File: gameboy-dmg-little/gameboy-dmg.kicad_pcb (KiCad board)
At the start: 2 copper layers, 82.5 x 87.5 mm, 83 parts, among them J1 Conn_01x02, J3 Conn_01x08, J5 Raspberry_Pi_2_3, J6 Conn_01x09, J7 USB_B_Micro, J8 Conn_01x02, P1 RK10J_POT, SW1 SW_DIP_x01, U1 MCP23017_SO, U2 TP4056, U3 FS312F-G, U4 FS8205, U5 MT3608, U6 PAM8302AAS

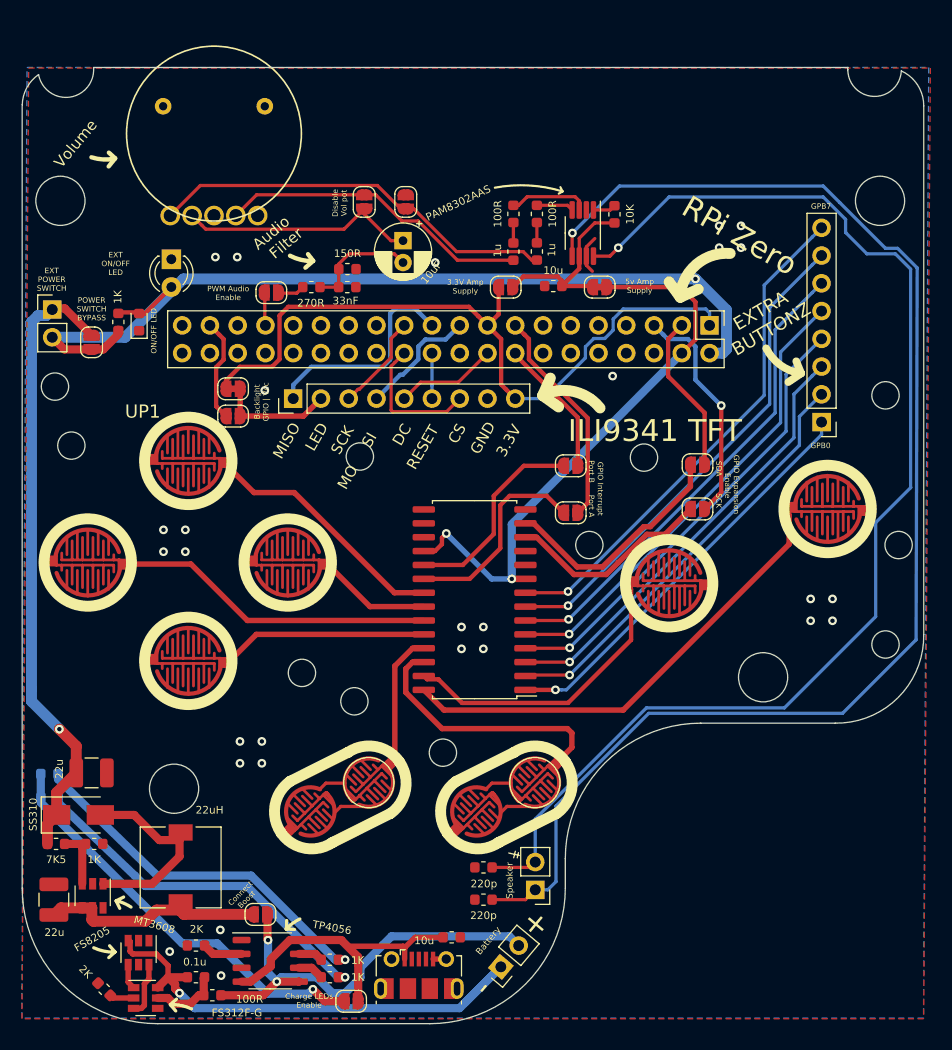
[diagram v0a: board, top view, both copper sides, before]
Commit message: Fixed up little board
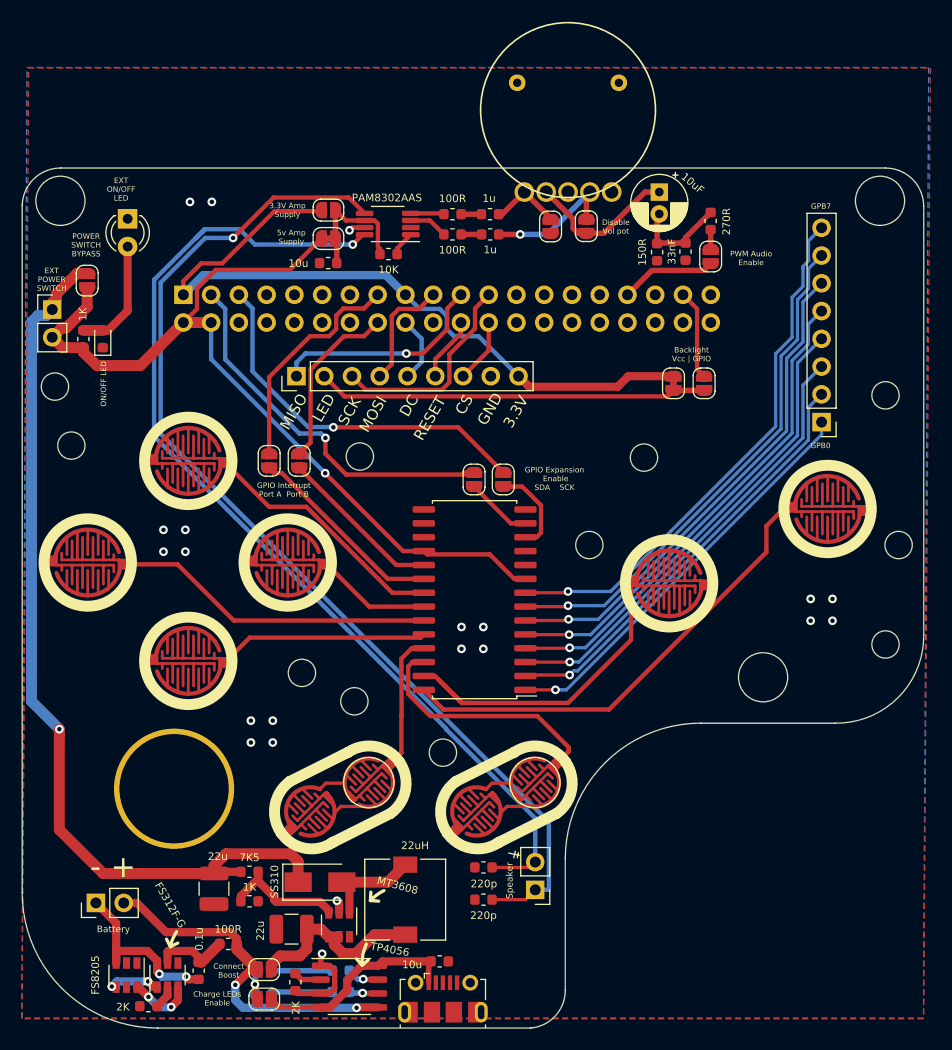
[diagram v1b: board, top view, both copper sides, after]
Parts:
- removed the G*** at (132.5, 122.9)
- removed the REF** at (83.5, 78.4)
- removed the REF** at (157.5, 78.4)
- added REF**: MountingHole_4.5mm, MountingHole:MountingHole_4.5mm, F.Cu at (157.5, 77.1)
- added REF**: MountingHole_4.5mm, MountingHole:MountingHole_4.5mm, F.Cu at (82.5, 77.1)
- J5, R4, R5: moved to B.Cu
- moved J5 48.2 mm to (93.8, 85.7)
- moved JP6 43.2 mm to (141.4, 93.8), turned to 270 degrees
- moved JP1 40.3 mm to (142.0, 82.2), turned to 90 degrees
- moved JP7 40.3 mm to (138.6, 93.8), turned to 270 degrees
- moved J8 37.5 mm to (85.8, 141.3), turned to 90 degrees
- moved R2 37.0 mm to (142.0, 79.0), turned to 270 degrees
- moved P1 32.5 mm to (128.9, 76.3)
- moved C1 31.1 mm to (139.7, 81.8), turned to 270 degrees
- moved R3 28.4 mm to (137.1, 81.8), turned to 90 degrees
- moved JP5 28.0 mm to (101.6, 100.9), turned to 270 degrees
- moved D4 26.6 mm to (101.1, 147.6)
- moved D3 26.6 mm to (101.1, 149.7)
- moved JP13 25.2 mm to (107.0, 80.5), turned to 0 degrees
- moved JP4 24.9 mm to (104.3, 100.9), turned to 270 degrees
- moved C2 23.9 mm to (137.3, 76.3)
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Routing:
- net +5V: track 132.7 -> 80.9 mm, vias 3 -> 1
- net Net-(D3-Pad2): track 38.2 -> 3.60 mm
- net /TP4056_LIPO_BOOST/BAT-: track 47.4 -> 16.5 mm, vias 1 -> 2
- net Net-(C8-Pad2): track 37.5 -> 6.72 mm
- net Net-(D4-Pad1): track 34.1 -> 5.46 mm, vias 1 -> 0
- net Net-(D3-Pad1): track 33.9 -> 5.56 mm, vias 1 -> 0
- net Net-(C10-Pad1): track 125.3 -> 98.3 mm
- net /TP4056_LIPO_BOOST/5V_BOOST: track 57.6 -> 84.4 mm
- net /TFT_BACKLIGHT: track 10.6 -> 35.8 mm
- net /GPIO_SDA_PI: track 14.7 -> 34.5 mm, vias 0 -> 1
- net Net-(C11-Pad1): track 114.7 -> 95.5 mm
- net Net-(C7-Pad1): track 28.7 -> 12.6 mm, vias 0 -> 1
- net /GPIO_SDA: track 21.8 -> 6.09 mm
- net /GPIO_SCK_PI: track 21.1 -> 34.3 mm
- net /GPIO_SCK: track 19.0 -> 8.27 mm
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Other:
- board size 82.5 x 87.5 mm -> 82.5 x 78.7 mm
- board text added: "Backlight Vcc | GPIO"
- board text added: "GPIO Interrupt Port A Port B"
- board text added: "MOSI"
- board text added: "Raspberry Pi Zero Gameboy DMG by Alex Hoffman"
- board text removed: "Audio Filter"
- board text removed: "Backlight GPIO | Vcc"
- board text removed: "EXTRA BUTTONZ"
- board text removed: "GPIO Interrupt Port B Port A"
- board text removed: "ILI9341 TFT"
- board text removed: "MO SI"
- board text removed: "RPi Zero"
- board text removed: "Raspberry Pi Zero Gameboy DMG Shield by Alex Hoffman"
- board text removed: "TUX"
- board text removed: "Volume"

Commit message: Little board gerbers
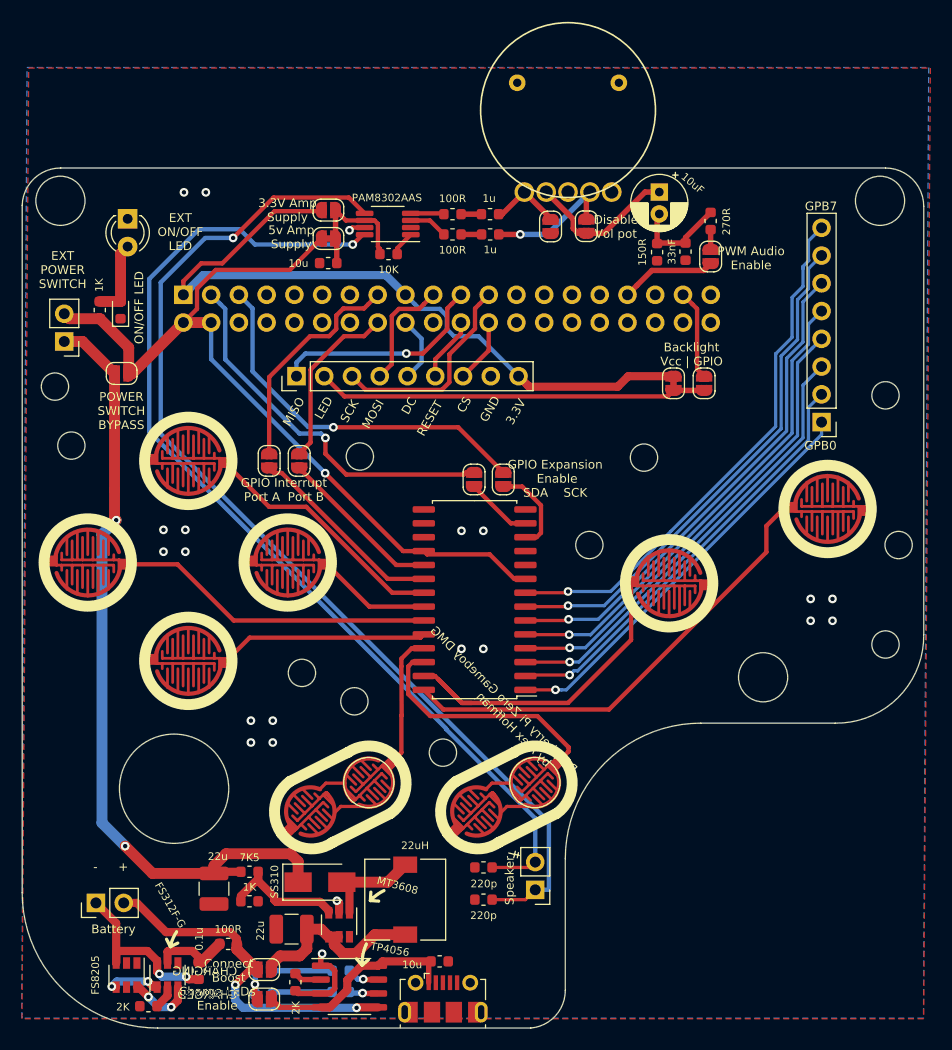
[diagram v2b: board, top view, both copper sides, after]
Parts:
- moved JP8 9.06 mm to (88.1, 92.9), turned to 0 degrees
- moved SW1 3.12 mm to (82.8, 90.0), turned to 180 degrees
- moved D1 3.11 mm to (88.0, 87.1)
- moved R1 3.05 mm to (86.1, 87.1)
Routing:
- net /TP4056_LIPO_BOOST/5V_BOOST: track 84.4 -> 73.3 mm, vias 1 -> 2
- net +5V: track 80.9 -> 76.3 mm
- net Net-(D1-Pad2): track 10.7 -> 7.19 mm
- net Net-(C11-Pad1): track 95.5 -> 94.7 mm
